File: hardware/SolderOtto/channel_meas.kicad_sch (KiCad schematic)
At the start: 57 parts, among them U901 OPA202, U902 LM358B, U903 74hc4053, U904 OPA202, U905 OPA202

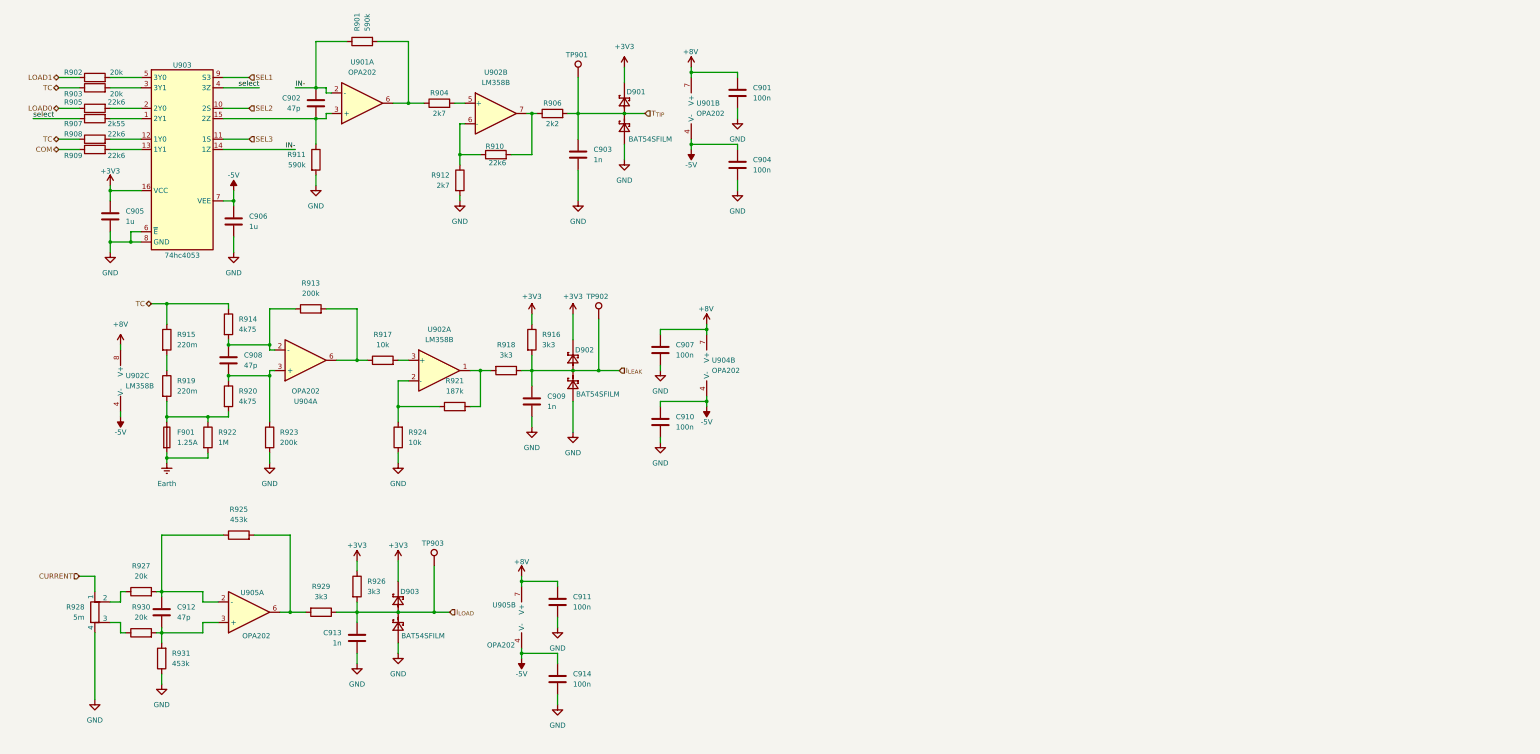
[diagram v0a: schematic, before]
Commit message: rework some shit
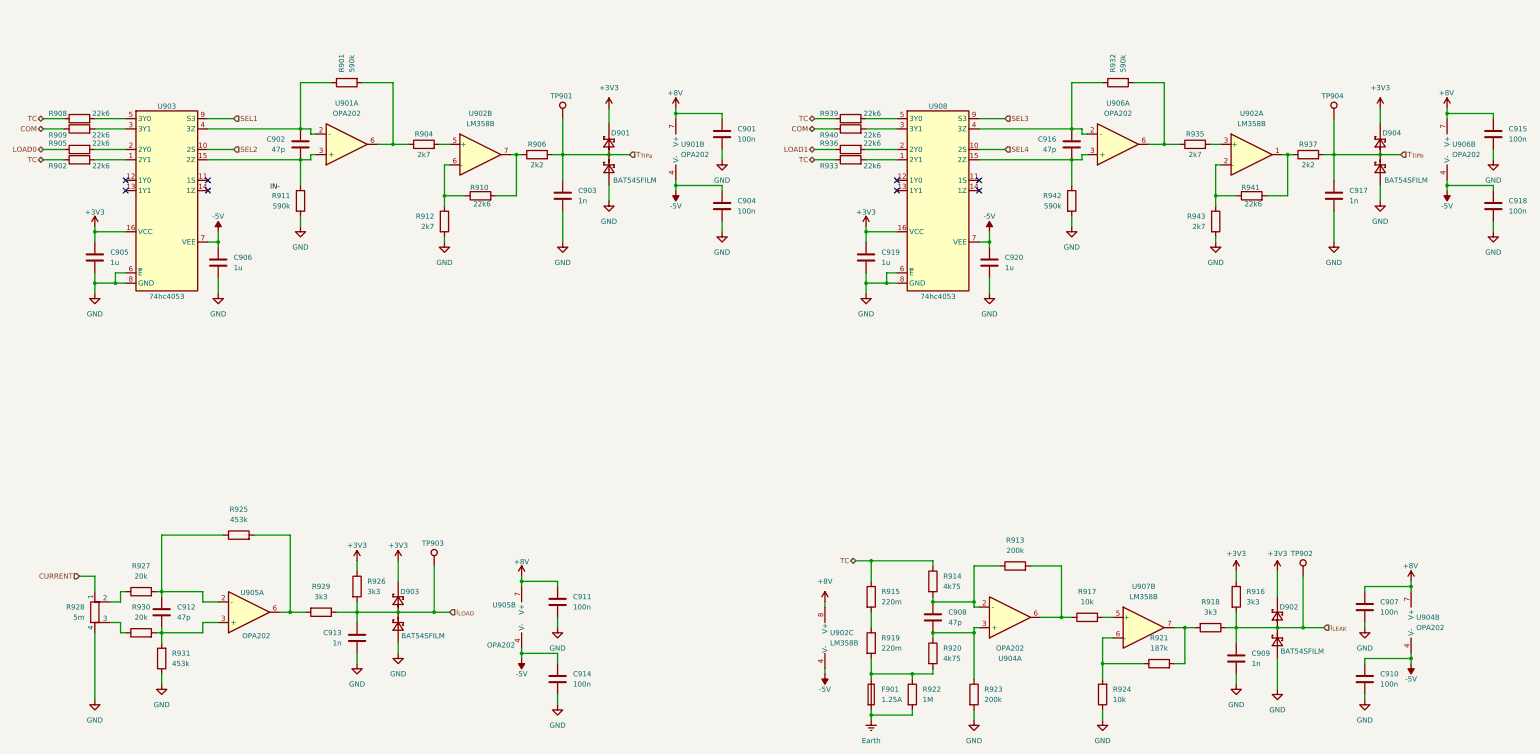
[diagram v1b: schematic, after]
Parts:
- removed R903: 20k, Resistor_SMD:R_0603_1608Metric, symbol Device:R
- removed R907: 2k55, Resistor_SMD:R_0603_1608Metric, symbol Device:R
- added C915, C918: 100n, Capacitor_SMD:C_0603_1608Metric, symbol Device:C
- added C916: 47p, Capacitor_SMD:C_0603_1608Metric, symbol Device:C
- added C917: 1n, Capacitor_SMD:C_0603_1608Metric, symbol Device:C
- added C919, C920: 1u, Capacitor_SMD:C_0603_1608Metric, symbol Device:C
- added D904: BAT54SFILM, Package_TO_SOT_SMD:SOT-23, symbol mylib_diodes:BAT54SFILM
- added R932, R942: 590k, Resistor_SMD:R_0603_1608Metric, symbol Device:R
- added R933, R936, R939, R940, R941: 22k6, Resistor_SMD:R_0603_1608Metric, symbol Device:R
- added R935, R943: 2k7, Resistor_SMD:R_0603_1608Metric, symbol Device:R
- added R937: 2k2, Resistor_SMD:R_0603_1608Metric, symbol Device:R
- added TP904: T_{TIP}, TestPoint:TestPoint_Keystone_5015_Micro-Minature, symbol Connector:TestPoint
- added U906: OPA202, Package_SO:SOIC-8_3.9x4.9mm_P1.27mm, symbol mylib_ic:OPA206
- added U907: LM358B, Package_SO:SOIC-8_3.9x4.9mm_P1.27mm, symbol Amplifier_Operational:LM358
- added U908: 74hc4053, Package_SO:TSSOP-16_4.4x5mm_P0.65mm, symbol mylib_ic:74hc4053
- R902: value 20k -> 22k6; Digikey P20.0KHCT-ND -> P22.6KHCT-ND
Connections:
- net +3V3: now also C919.1, D904.2, U908.16 (VCC)
- net +8V: now also C915.1, U906.7 (V+)
- net -5V: now also C918.1, C920.1, U906.4 (V-), U908.7 (VEE)
- net COM: now also R940.1
- net GND: now also C915.2, C917.2, C918.2, C919.2, C920.2, D904.1, R942.2, R943.2, U908.6 (~{E}), U908.8 (GND)
- net IN-: no longer C902.1, R901.1, U901.2 (-), U903.14 (1Z)
- net LOAD1: now also R936.1; no longer R902.1
- net SEL3: now also U908.9 (S3); no longer U903.11 (1S)
- net TC: now also R902.1, R933.1, R939.1
- net at R918.2, R921.2: now also U907.7; no longer U902.1
- net at U903.1 (2Y1): now also R902.2
- net at U903.12 (1Y0): no longer R908.2
- net at U903.13 (1Y1): no longer R909.2
- net at U903.3 (3Y1): now also R909.2
- net at U903.5 (3Y0): now also R908.2; no longer R902.2
- net at R921.1, R924.2: now also U907.6 (-); no longer U902.2 (-)
- net at U902.3 (+): now also R935.2; no longer R917.2
- net T_{TIP} renamed T_{TIP}_{a}
- net select: no longer names the net of U903.4 (3Z)
- net select: now also C902.1, R901.1, U901.2 (-)
- new net: C916.2, R942.1, U906.3 (+), U908.15 (2Z)
- new net: R936.2, U908.2 (2Y0)
- new net: R940.2, U908.3 (3Y1)
- new net: R933.2, U908.1 (2Y1)
- new net: C916.1, R932.1, U906.2 (-), U908.4 (3Z)
- new net: R939.2, U908.5 (3Y0)
- new net: R937.1, R941.2, U902.1
- new net: R941.1, R943.1, U902.2 (-)
- new net: R932.2, R935.1, U906.6
- new net: R917.2, U907.5 (+)
- new net: U906.1 (NC), U906.5 (NC), U906.8 (NC)
- new net SEL4: U908.10 (2S)
- new net T_{TIP}_{b}: C917.1, D904.3, R937.2, TP904.1
- no-connect marks 0 -> 8
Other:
- moved on the sheet: C901, C902, C903, C904, C905, C906, C907, C908, C909, C910, D901, D902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
